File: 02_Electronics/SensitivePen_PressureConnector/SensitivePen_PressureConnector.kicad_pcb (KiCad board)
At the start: 2 copper layers, 5 x 8.8 mm, 2 parts, among them J1 Conn_01x02, J2 Conn_01x02

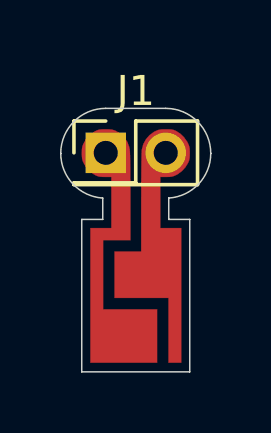
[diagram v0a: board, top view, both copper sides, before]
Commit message: update
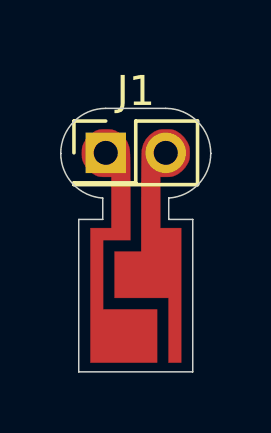
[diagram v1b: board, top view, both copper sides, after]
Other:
- outline, holes or cut-outs redrawn
